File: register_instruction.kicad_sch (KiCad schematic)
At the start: 18 parts, among them U26 74LS573, U27 74LS245

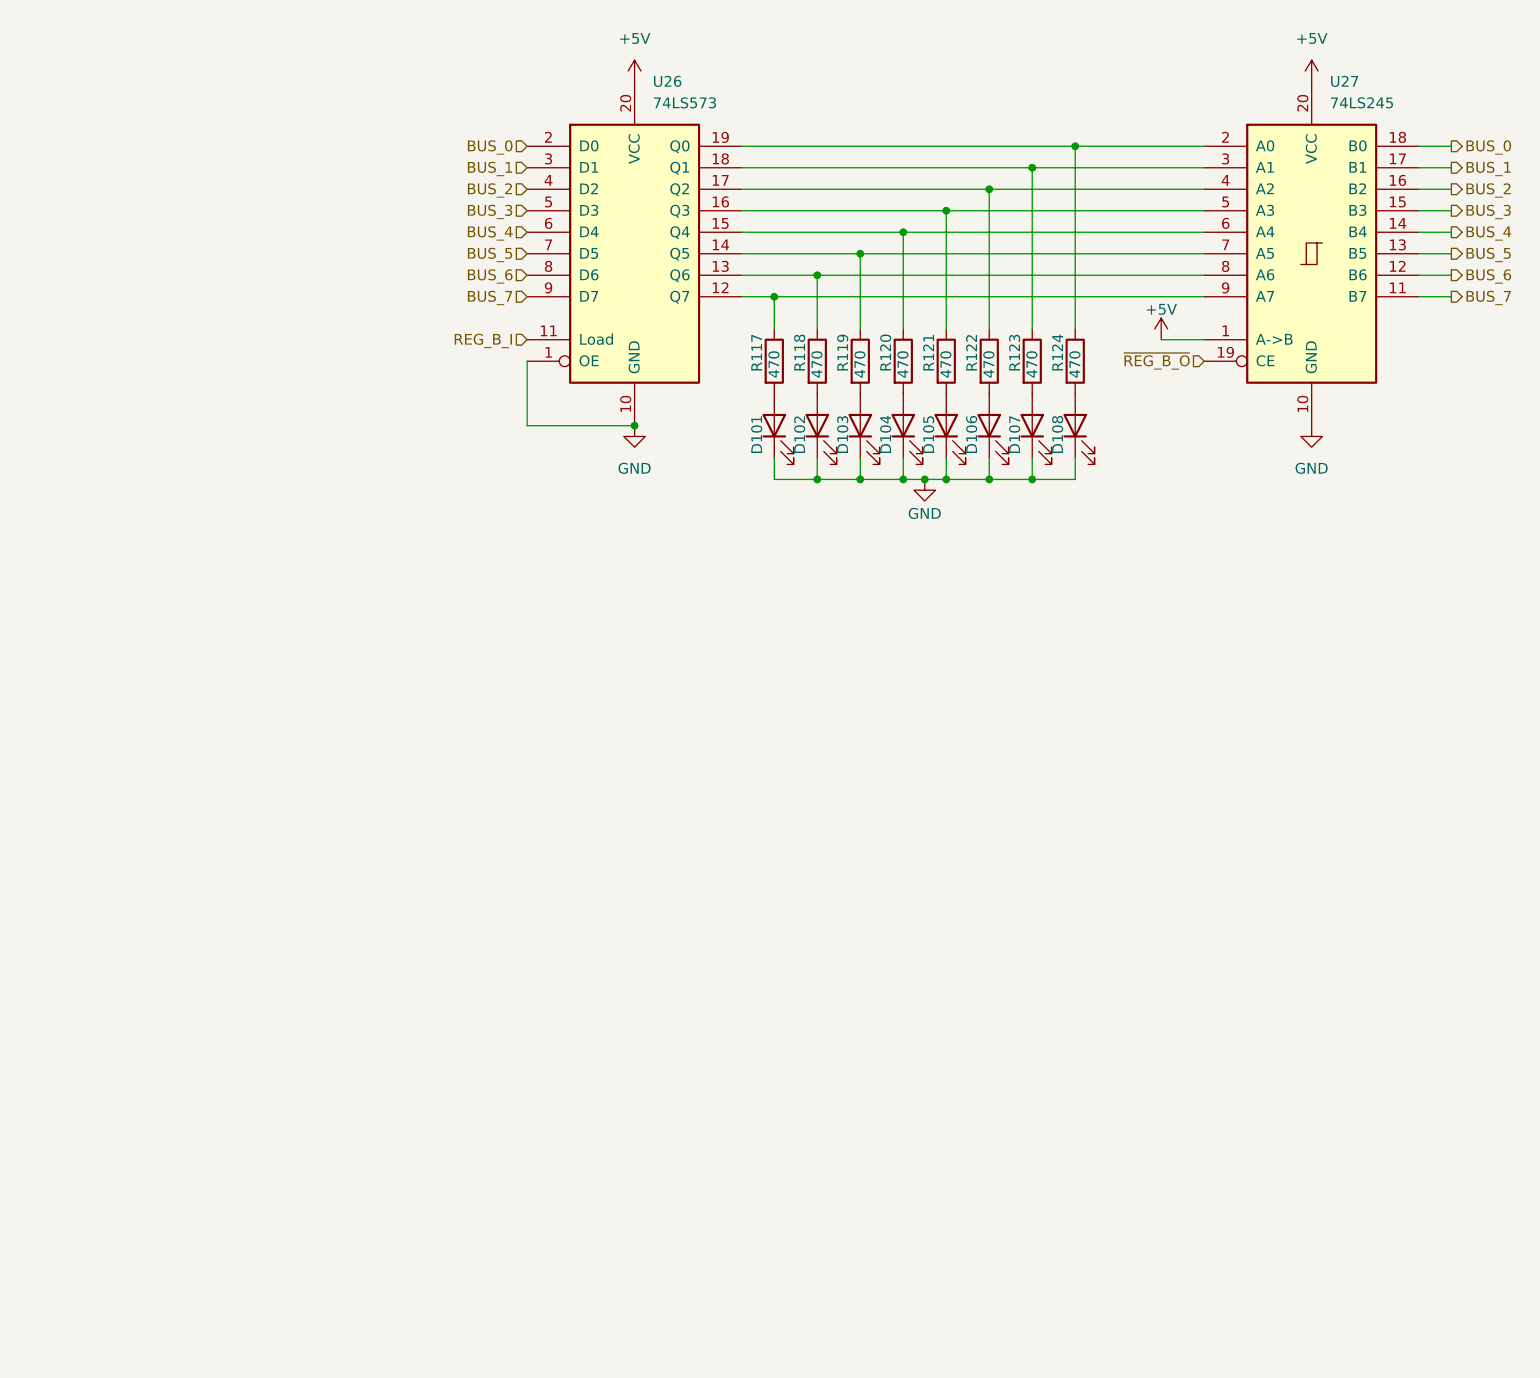
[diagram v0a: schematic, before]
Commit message: chore: sync files
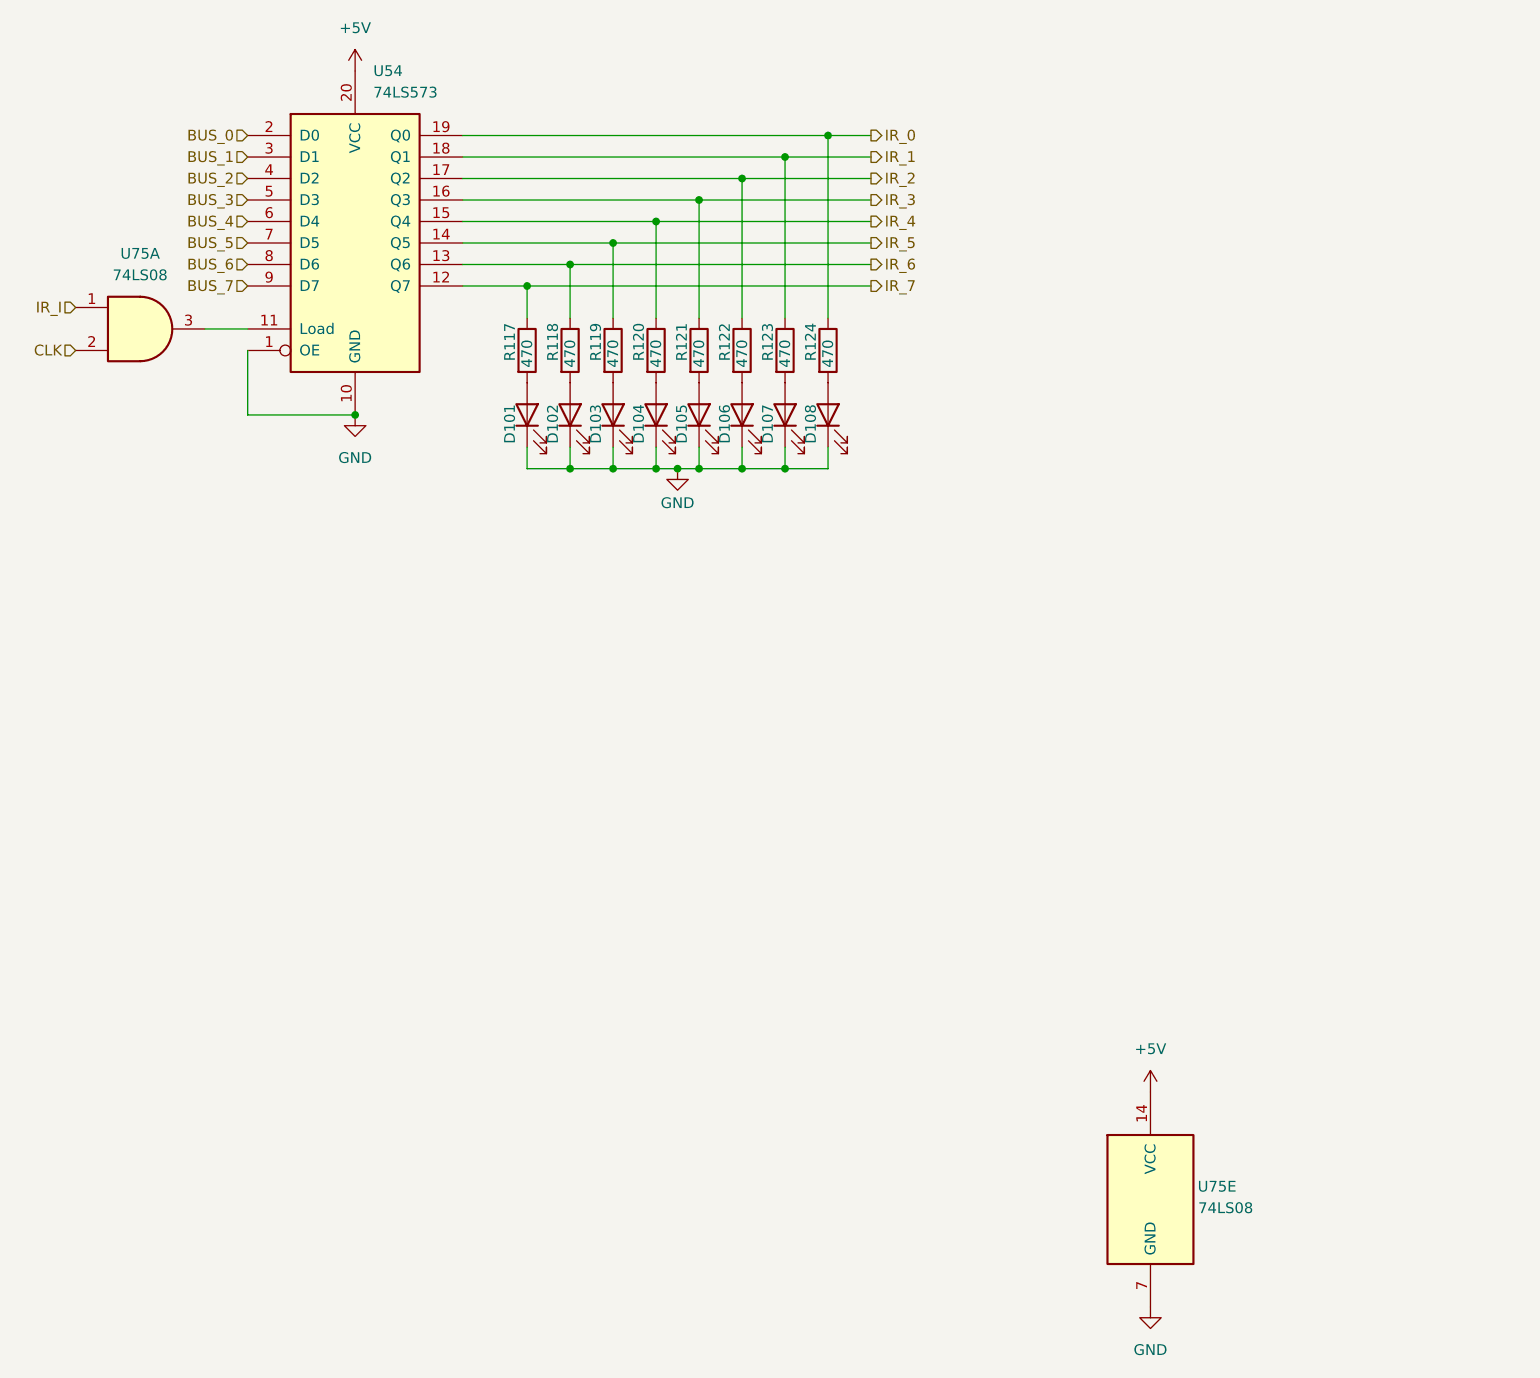
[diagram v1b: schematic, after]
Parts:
- removed U26: 74LS573, symbol 74xx:74LS573
- removed U27: 74LS245, symbol 74xx:74LS245
- added U54: 74LS573, Package_DIP:DIP-20_W7.62mm_Socket, symbol 74xx:74LS573
- added U75: 74LS08, Package_DIP:DIP-14_W7.62mm_Socket, symbol 74xx:74LS08
- D101, D102, D103, D104, D105, D106, D107, D108: footprint (none) -> LED_SMD:LED_0805_2012Metric
- R117, R118, R119, R120, R121, R122, R123, R124: footprint (none) -> Resistor_SMD:R_0805_2012Metric
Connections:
- net +5V: now also U54.20 (VCC), U75.14 (VCC)
- net BUS_0: now also U54.2 (D0)
- net BUS_1: now also U54.3 (D1)
- net BUS_2: now also U54.4 (D2)
- net BUS_3: now also U54.5 (D3)
- net BUS_4: now also U54.6 (D4)
- net BUS_5: now also U54.7 (D5)
- net BUS_6: now also U54.8 (D6)
- net BUS_7: now also U54.9 (D7)
- net GND: now also U54.1 (OE), U54.10 (GND), U75.7 (GND)
- net IR_7: now reaches R117.1
- net IR_7: now also U54.12 (Q7)
- net IR_6: now reaches R118.1
- net IR_6: now also U54.13 (Q6)
- net IR_5: now reaches R119.1
- net IR_5: now also U54.14 (Q5)
- net IR_4: now reaches R120.1
- net IR_4: now also U54.15 (Q4)
- net IR_3: now reaches R121.1
- net IR_3: now also U54.16 (Q3)
- net IR_2: now reaches R122.1
- net IR_2: now also U54.17 (Q2)
- net IR_1: now reaches R123.1
- net IR_1: now also U54.18 (Q1)
- net IR_0: now reaches R124.1
- net IR_0: now also U54.19 (Q0)
- new net: U54.11 (Load), U75.3
- new net CLK: U75.2
- new net IR_I: U75.1
